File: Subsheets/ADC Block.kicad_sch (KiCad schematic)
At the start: 26 parts, among them U140 AD7490SRUZ-EP-RL7, U141 REF3425SQDBVRQ1, U49 AD7490SRUZ-EP-RL7

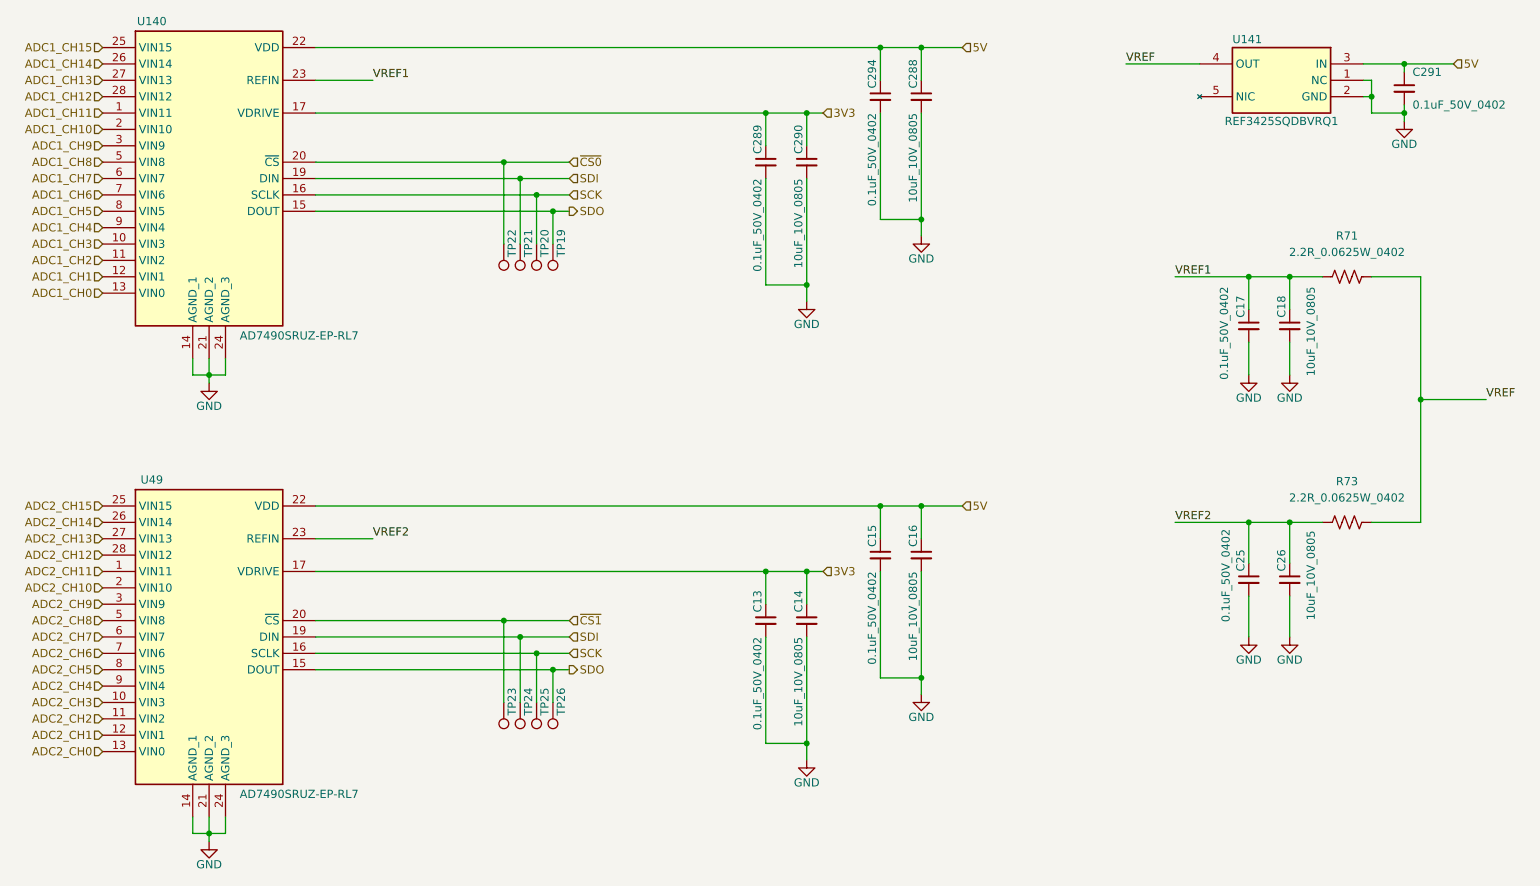
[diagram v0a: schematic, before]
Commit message: Schematic Update-1.1
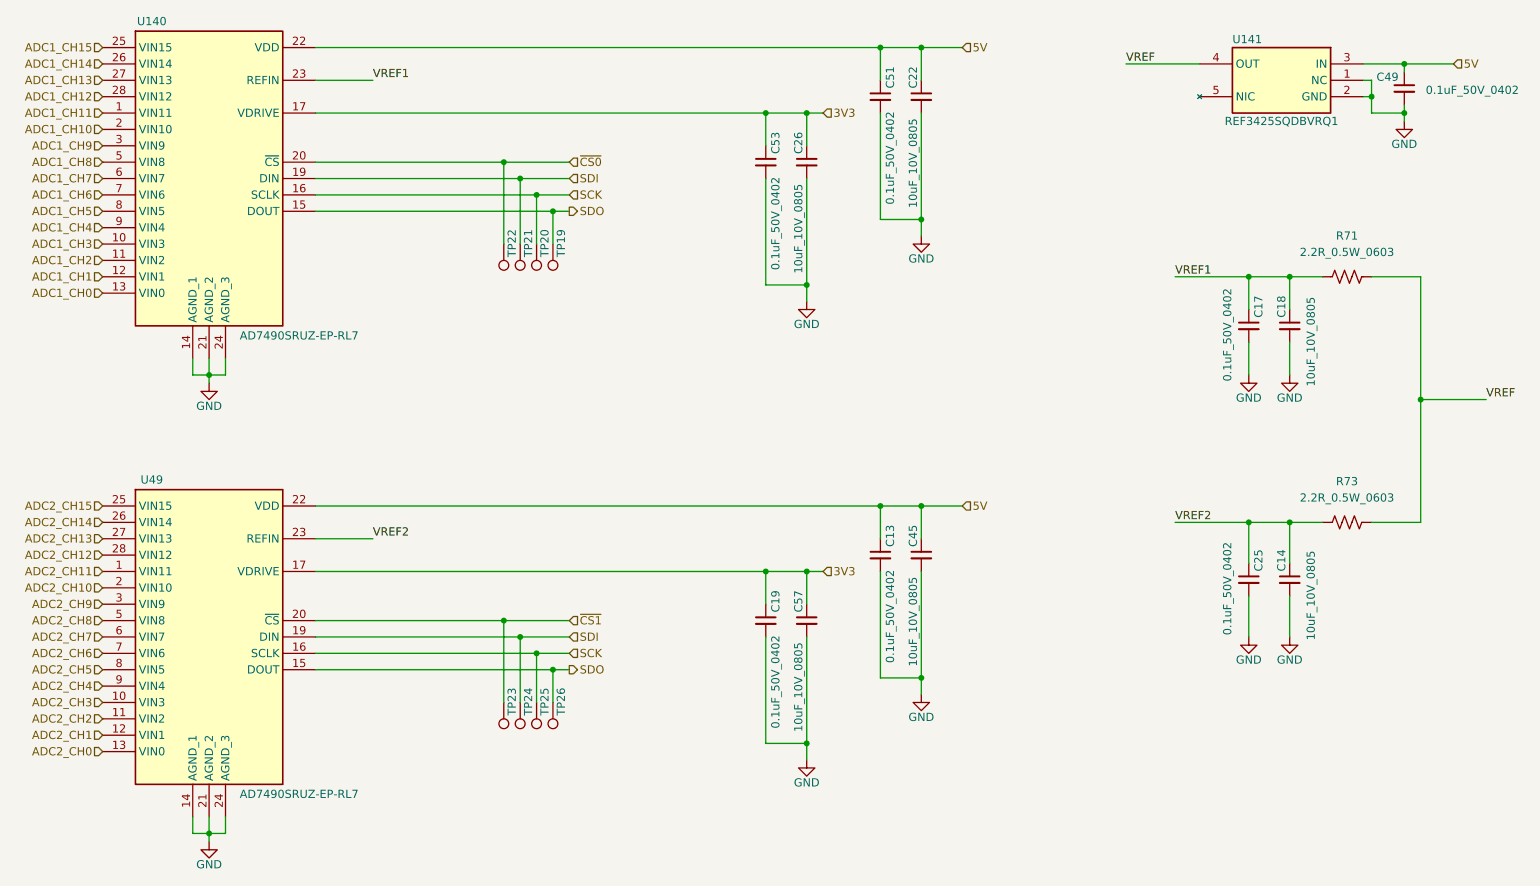
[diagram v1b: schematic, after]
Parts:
- removed C15, C289, C291, C294: 0.1uF_50V_0402, Pixxel_Capacitors:CAP0402, symbol Device:C_Small
- removed C16, C288, C290: 10uF_10V_0805, symbol Device:C_Small
- added C19, C49, C51, C53: 0.1uF_50V_0402, Pixxel_Capacitors:CAP0402, symbol Device:C_Small
- added C22, C45, C57: 10uF_10V_0805, Pixxel_Capacitors:CAP0805, symbol Device:C_Small
- C13, C17, C25: Manufacturer_Part_Number GCM155R71H104KE02J -> (none); Vendor_Part_Number 490-14514-2-ND -> (none)
- C14, C18, C26: footprint (none) -> Pixxel_Capacitors:CAP0805; Manufacturer Murata Electronics -> (none); Manufacturer Name (none) -> Murata Electronics; Manufacturer_Part_Number GCM21BR71A106KE22L -> (none); Mass (grams) 0.001 -> (none); Power Dissipation (W) NA -> (none); Price(INR) (none) -> 34.97; RQjC (C/W) NA -> (none); Temp_max (C) 105 -> 125; Vendor (none) -> Digikey; Vendor Part Number (none) -> 490-10674-2-ND
- R71, R73: value 2.2R_0.0625W_0402 -> 2.2R_0.5W_0603; footprint (none) -> Pixxel_Resistors:RES0603; Manufacturer Name (none) -> Vishay Dale; Manufacturer Part Number (none) -> TNPW06032R20DEEA; Price(INR) (none) -> 16.07; Temp_max (C) (none) -> 175; Temp_min (C) (none) -> -55; Vendor (none) -> Digikey; Vendor Part Number (none) -> 541-TNPW06032R20DEEATR-ND
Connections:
- net 3V3: now also C26.1, C19.1, C53.1, C57.1; no longer C13.1, C14.1
- net 5V: now also C13.1, C22.1, C45.1, C49.1, C51.1
- net GND: now also C19.2, C22.2, C45.2, C49.2, C51.2, C53.2, C57.2
- net VREF2: now also C14.1; no longer C26.1
